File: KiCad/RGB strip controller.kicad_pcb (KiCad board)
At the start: 2 copper layers, 11.7 x 33.8 mm, 22 parts, among them J1 USB_C_Receptacle_USB2.0, J2 Conn_01x03, Q1 BC847, Q2 BC847, U1 ESP-01, U2 SPX3819M5-L-3-3, U3 TC7SZ125FU, U4 CH340G, Y1 12M

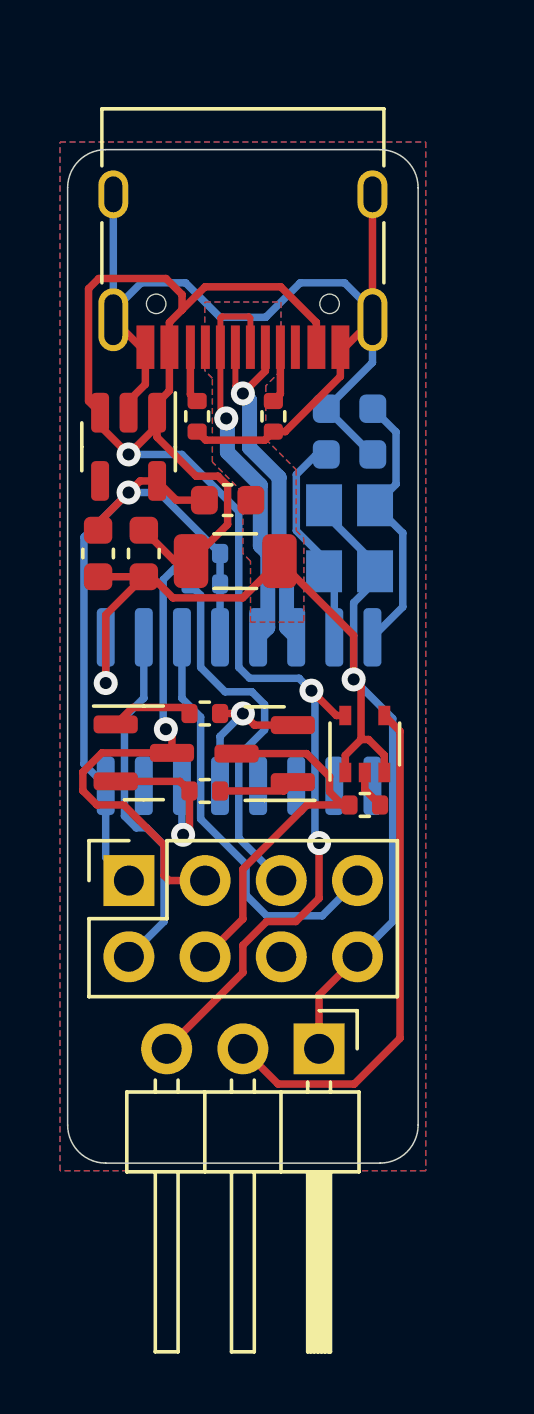
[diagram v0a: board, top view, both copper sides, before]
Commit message: Finalize v4 PCB
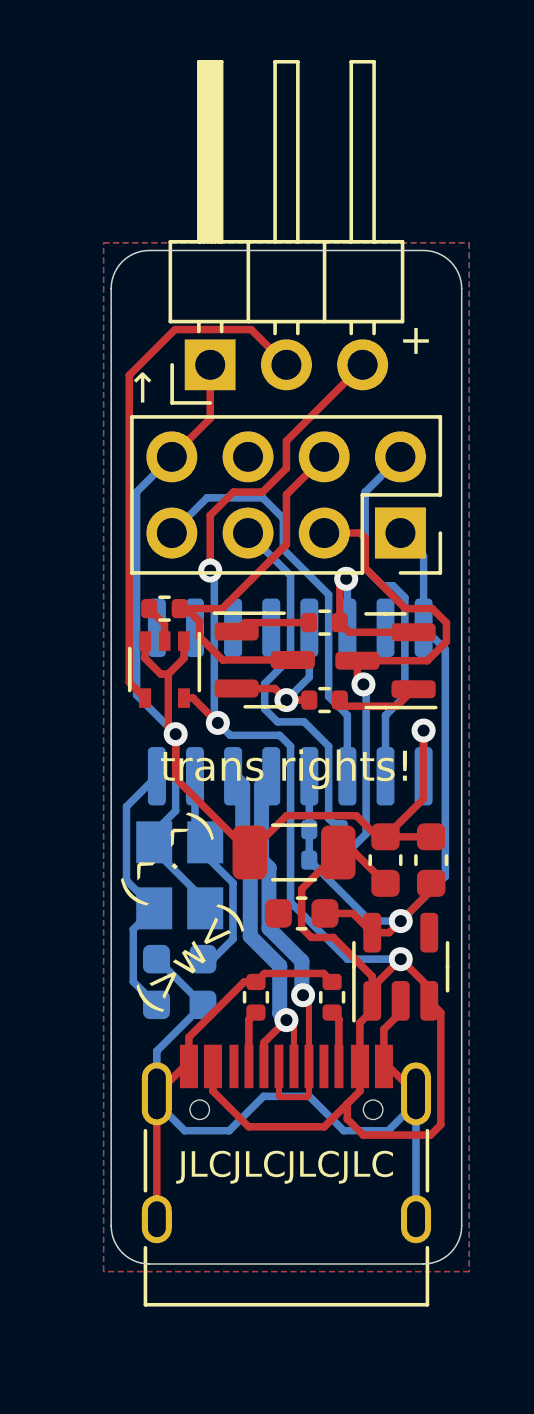
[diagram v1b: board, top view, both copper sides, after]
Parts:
- added G***: umbreon_2layer_6mm, _Project:umbreon_2layer_6mm, B.Cu at (170.4, 135.4)
- added REF**: OSHW-Logo2_7.3x6mm_SilkScreen, Symbol:OSHW-Logo2_7.3x6mm_SilkScreen, B.Cu at (171.2, 129.5)
- moved J1 32.1 mm to (170.6, 136.7), turned to 0 degrees
- moved J2 23.1 mm to (168.1, 109.3), turned to 90 degrees
- moved C6 20.7 mm to (167.1, 130.6), turned to 0 degrees
- moved R2 19.9 mm to (172.1, 130.4), turned to 90 degrees
- moved U2 19.6 mm to (174.4, 129.3), turned to 90 degrees
- moved R3 19.4 mm to (169.6, 130.4), turned to 90 degrees
- moved C5 17.8 mm to (167.1, 129.1), turned to 180 degrees
- moved C4 15.1 mm to (175.4, 125.8), turned to 90 degrees
- moved U1 14.7 mm to (174.4, 114.9), turned to -90 degrees
- moved C3 14.0 mm to (171.1, 127.6), turned to 180 degrees
- moved C2 13.0 mm to (173.9, 125.8), turned to 90 degrees
- moved Y1 12.6 mm to (167.1, 126.3), turned to -90 degrees
- moved R7 11.0 mm to (171.9, 125.8), turned to 180 degrees
- moved C1 9.91 mm to (170.9, 125.5), turned to 180 degrees
- moved R4 9.35 mm to (166.6, 117.4), turned to 0 degrees
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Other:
- board text added: "(>w<)"
- board text added: "(^.^)"
- board text added: "+"
- board text added: "2022.10.04"
- board text added: "<.<"
- board text added: ">.>"
- board text added: "JLCJLCJLCJLC"
- board text added: "archive.eritbh.me/rgb"
- board text added: "trans rights!"
- board text added: "v4"
- board text added: "→"
